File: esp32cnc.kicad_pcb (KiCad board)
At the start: 2 copper layers, 88.3 x 113.7 mm, 25 parts, among them J1 Barrel_Jack, J2 USB_B_Micro, J3 Micro_SD_Card_Det1, J4 Screw_Terminal_01x04, J5 Screw_Terminal_01x04, J6 Screw_Terminal_01x04, J7 Screw_Terminal_01x02, U1 ESP32-WROOM-32, U2 OKI-78SR-3.3_1.5-W36-C, U3 CH330N, U4 DRV8871DDA

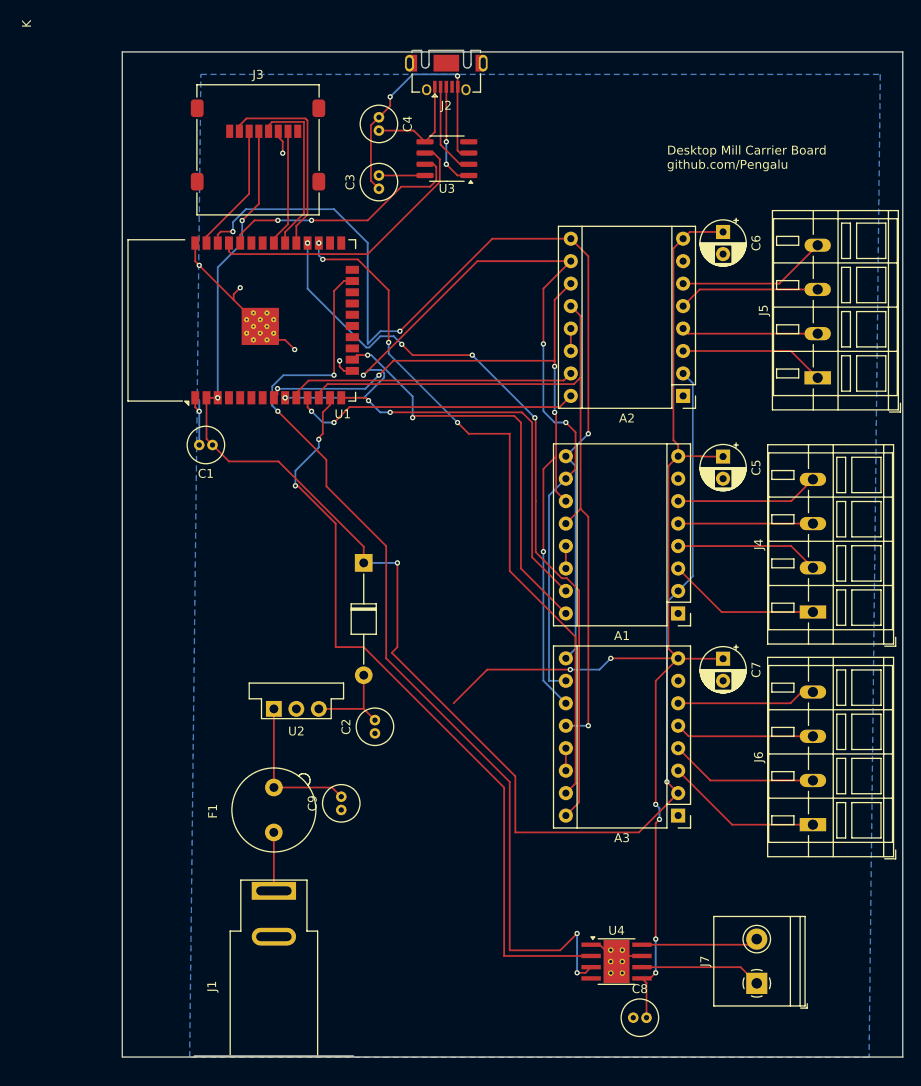
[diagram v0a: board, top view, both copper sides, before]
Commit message: Init
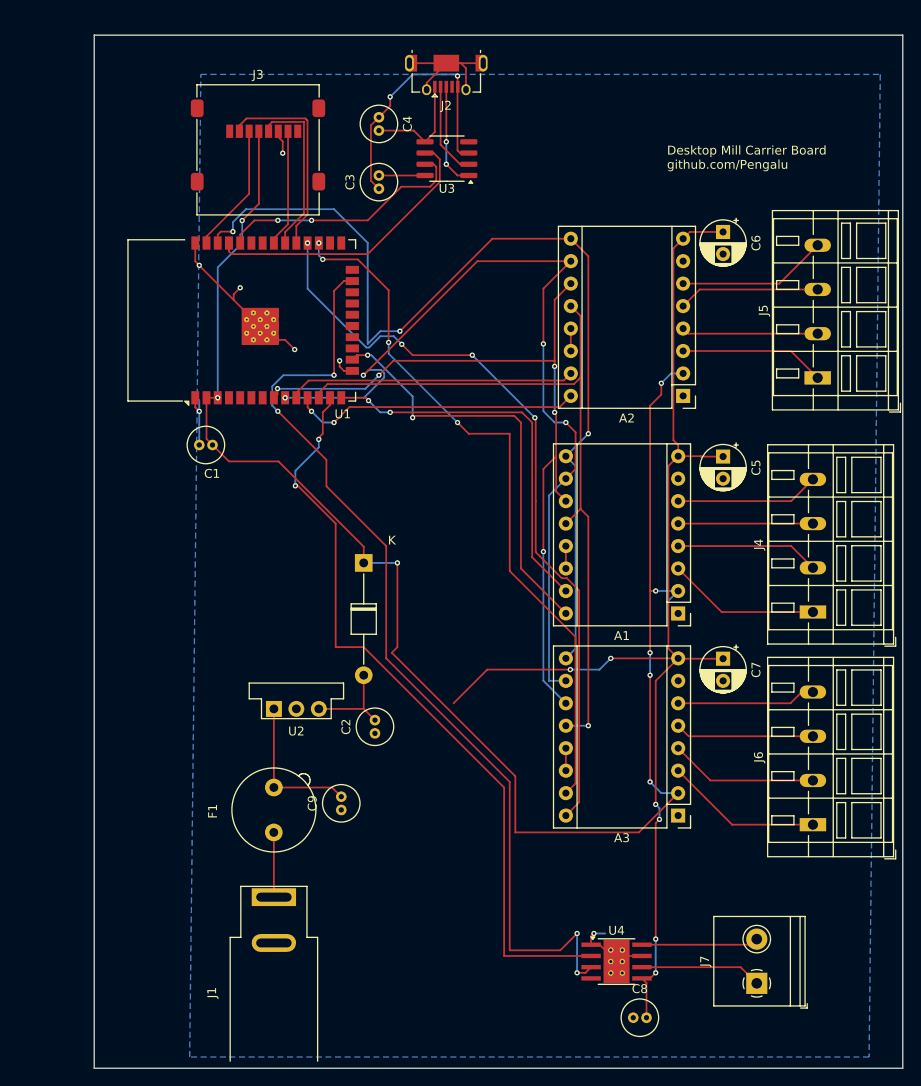
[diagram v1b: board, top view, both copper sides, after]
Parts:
- moved J1 0.71 mm to (121.9, 122.9)
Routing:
- net unconnected-(J2-Shield-Pad6)_4: track 0.00 -> 16.3 mm
- net GND: track 63.1 -> 74.9 mm, vias 8 -> 9
- net +3.3V: track 173.7 -> 181.3 mm, vias 4 -> 8
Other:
- board size 88.3 x 113.7 mm -> 91.4 x 116.8 mm
